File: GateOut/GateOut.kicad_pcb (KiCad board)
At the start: 2 copper layers, 20.3 x 10.2 mm, 16 parts, among them J1 Conn_01x04, J2 Conn_01x04, U1 LM358

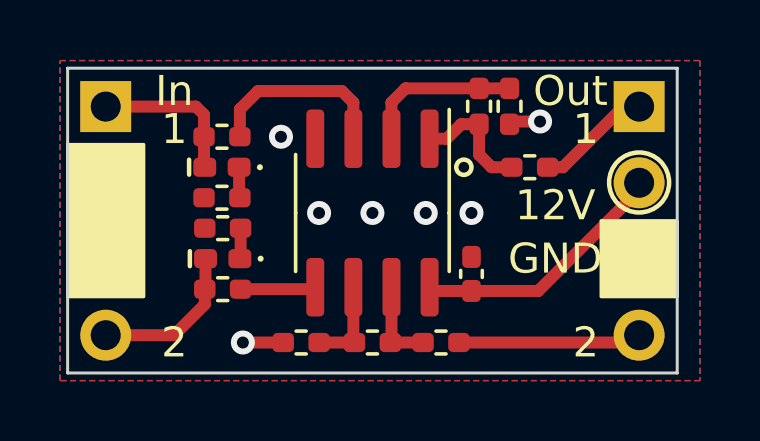
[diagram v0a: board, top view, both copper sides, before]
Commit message: GateOutのPCBのささかいな更新
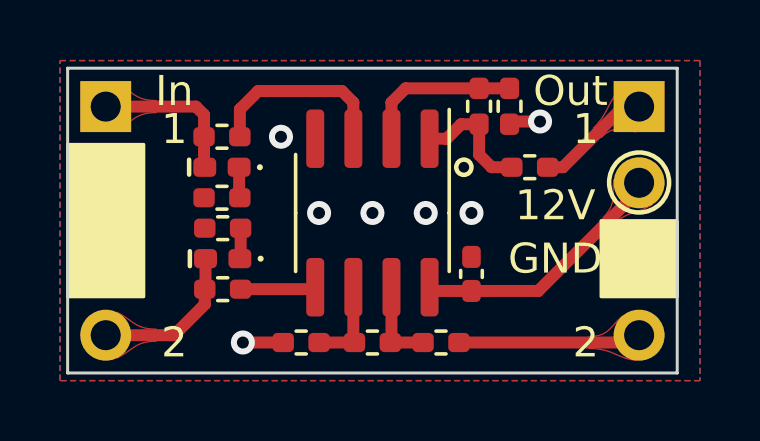
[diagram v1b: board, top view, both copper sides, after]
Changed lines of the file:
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@@
   (segment (start 106.147 79.477) (end 106.172 79.502) (width 0.4) (layer "F.Cu") (net 4))
   (segment (start 106.147 77.749) (end 105.878 77.48) (width 0.4) (layer "F.Cu") (net 4))
-  (segment (start 102.88 77.47) (end 102.87 77.48) (width 0.4) (layer "F.Cu") (net 4))
   (segment (start 106.147 78.486) (end 106.147 79.477) (width 0.4) (layer "F.Cu") (net 4))
   (segment (start 106.147 78.486) (end 106.147 77.749) (width 0.4) (layer "F.Cu") (net 4))
@@
   (segment (start 114.6435 85.344) (end 120.406 85.344) (width 0.4) (layer "F.Cu") (net 14))
   (segment (start 120.406 85.344) (end 120.65 85.1) (width 0.4) (layer "F.Cu") (net 14))
+  (zone (net 13) (net_name "/out1") (layer "F.Cu") (hatch edge 0.508)
+    (priority 16962)
+    (connect_pads yes (clearance 0))
+    (min_thickness 0.0254) (filled_areas_thickness no)
+    (fill yes (thermal_gap 0.508) (thermal_bridge_width 0.508))
+    (polygon
+      (pts
+        (xy 119.382468 78.512375)
+        (xy 119.503927 78.40324)
+        (xy 119.617271 78.325793)
+        (xy 119.725231 78.275685)
+        (xy 119.830538 78.248568)
+        (xy 119.935925 78.240095)
+        (xy 120.044122 78.245916)
+        (xy 120.157862 78.261683)
+        (xy 120.279875 78.283049)
+        (xy 120.412893 78.305665)
+        (xy 120.559649 78.325184)
+        (xy 121.050024 77.336455)
+        (xy 120.042885 76.885096)
+        (xy 119.910756 77.030949)
+        (xy 119.808694 77.164946)
+        (xy 119.728575 77.290582)
+        (xy 119.662272 77.411352)
+        (xy 119.601661 77.530752)
+        (xy 119.538618 77.652277)
+        (xy 119.465018 77.779422)
+        (xy 119.372735 77.915683)
+        (xy 119.253646 78.064554)
+        (xy 119.099625 78.229532)
+      )
+    )
+  )
+  (zone (net 6) (net_name "/in2") (layer "F.Cu") (hatch edge 0.508)
+    (priority 16962)
+    (connect_pads yes (clearance 0))
+    (min_thickness 0.0254) (filled_areas_thickness no)
+    (fill yes (thermal_gap 0.508) (thermal_bridge_width 0.508))
+    (polygon
+      (pts
+        (xy 104.56 84.9)
+        (xy 104.363815 84.891521)
+        (xy 104.20108 84.867344)
+        (xy 104.064604 84.829353)
+        (xy 103.947195 84.779433)
+        (xy 103.841665 84.719471)
+        (xy 103.740821 84.65135)
+        (xy 103.637473 84.576957)
+        (xy 103.524432 84.498178)
+        (xy 103.394506 84.416897)
+        (xy 103.240506 84.335)
+        (xy 102.445 85.1)
+        (xy 103.240506 85.865)
+        (xy 103.394506 85.783102)
+        (xy 103.524432 85.701821)
+        (xy 103.637473 85.623042)
+        (xy 103.740821 85.548649)
+        (xy 103.841665 85.480528)
+        (xy 103.947195 85.420566)
+        (xy 104.064604 85.370646)
+        (xy 104.20108 85.332655)
+        (xy 104.363815 85.308478)
+        (xy 104.56 85.3)
+      )
+    )
+  )
+  (zone (net 4) (net_name "/in1") (layer "F.Cu") (hatch edge 0.508)
+    (priority 16962)
+    (connect_pads yes (clearance 0))
+    (min_thickness 0.0254) (filled_areas_thickness no)
+    (fill yes (thermal_gap 0.508) (thermal_bridge_width 0.508))
+    (polygon
+      (pts
+        (xy 104.56 77.28)
+        (xy 104.363815 77.271521)
+        (xy 104.20108 77.247344)
+        (xy 104.064604 77.209353)
+        (xy 103.947195 77.159433)
+        (xy 103.841665 77.099471)
+        (xy 103.740821 77.03135)
+        (xy 103.637473 76.956957)
+        (xy 103.524432 76.878178)
+        (xy 103.394506 76.796897)
+        (xy 103.240506 76.715)
+        (xy 102.445 77.48)
+        (xy 103.240506 78.245)
+        (xy 103.394506 78.163102)
+        (xy 103.524432 78.081821)
+        (xy 103.637473 78.003042)
+        (xy 103.740821 77.928649)
+        (xy 103.841665 77.860528)
+        (xy 103.947195 77.800566)
+        (xy 104.064604 77.750646)
+        (xy 104.20108 77.712655)
+        (xy 104.363815 77.688478)
+        (xy 104.56 77.68)
+      )
+    )
+  )
+  (zone (net 14) (net_name "/out2") (layer "F.Cu") (hatch edge 0.508)
+    (priority 16962)
+    (connect_pads yes (clearance 0))
+    (min_thickness 0.0254) (filled_areas_thickness no)
+    (fill yes (thermal_gap 0.508) (thermal_bridge_width 0.508))
+    (polygon
+      (pts
+        (xy 118.976 85.544)
+        (xy 119.193325 85.552029)
+        (xy 119.374934 85.574303)
+        (xy 119.528909 85.608101)
+        (xy 119.663334 85.6507)
+        (xy 119.78629 85.699379)
+        (xy 119.905861 85.751416)
+        (xy 120.030129 85.804089)
+        (xy 120.167178 85.854678)
+        (xy 120.32509 85.90046)
+        (xy 120.511949 85.938714)
+        (xy 121.057509 84.97933)
+        (xy 120.077536 84.471682)
+        (xy 119.963368 84.582297)
+        (xy 119.865715 84.686655)
+        (xy 119.77872 84.783485)
+        (xy 119.696522 84.871521)
+        (xy 119.613263 84.949493)
+        (xy 119.523085 85.016133)
+        (xy 119.420128 85.070172)
+        (xy 119.298534 85.110341)
+        (xy 119.152444 85.135374)
+        (xy 118.976 85.144)
+      )
+    )
+  )
+  (zone (net 1) (net_name "+12V") (layer "F.Cu") (hatch edge 0.508)
+    (priority 16962)
+    (connect_pads yes (clearance 0))
+    (min_thickness 0.0254) (filled_areas_thickness no)
+    (fill yes (thermal_gap 0.508) (thermal_bridge_width 0.508))
+    (polygon
+      (pts
+        (xy 119.723691 81.473152)
+        (xy 119.87883 81.329649)
+        (xy 120.019563 81.221493)
+        (xy 120.149718 81.141357)
+        (xy 120.273122 81.081916)
+        (xy 120.393601 81.035844)
+        (xy 120.514984 80.995814)
+        (xy 120.641095 80.954502)
+        (xy 120.775764 80.904581)
+        (xy 120.922816 80.838726)
+        (xy 121.08608 80.749611)
+        (xy 120.883283 79.664749)
+        (xy 119.807176 79.909791)
+        (xy 119.791394 80.072406)
+        (xy 119.785463 80.218164)
+        (xy 119.783949 80.350505)
+        (xy 119.781422 80.472871)
+        (xy 119.772451 80.588704)
+        (xy 119.751605 80.701444)
+        (xy 119.713453 80.814533)
+        (xy 119.652563 80.931413)
+        (xy 119.563505 81.055524)
+        (xy 119.440848 81.190309)
+      )
+    )
+  )
   (zone (net 2) (net_name "GND") (layers F&B.Cu) (hatch edge 0.508)
     (connect_pads (clearance 0.508))
